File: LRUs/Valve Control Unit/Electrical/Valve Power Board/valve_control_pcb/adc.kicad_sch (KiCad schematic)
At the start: 8 parts, among them U37 AD7689BCP

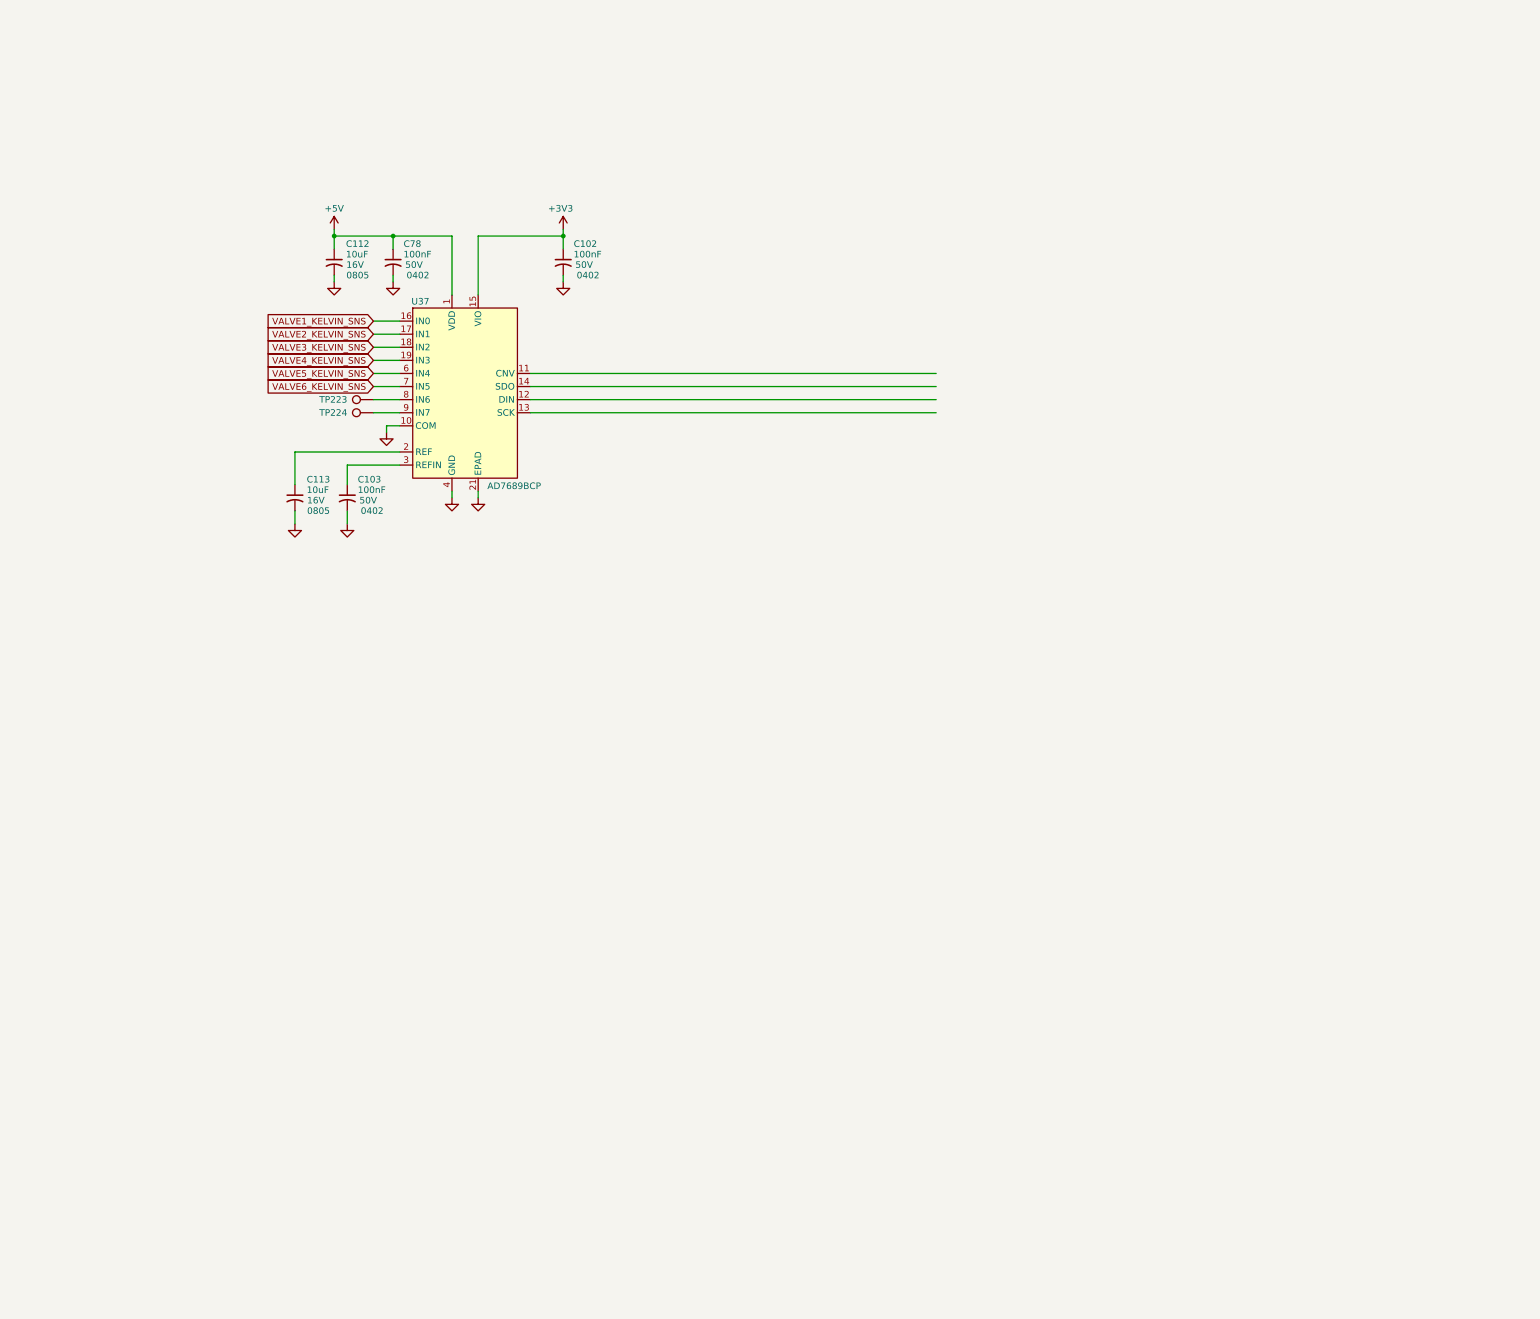
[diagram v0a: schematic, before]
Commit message: Committttt
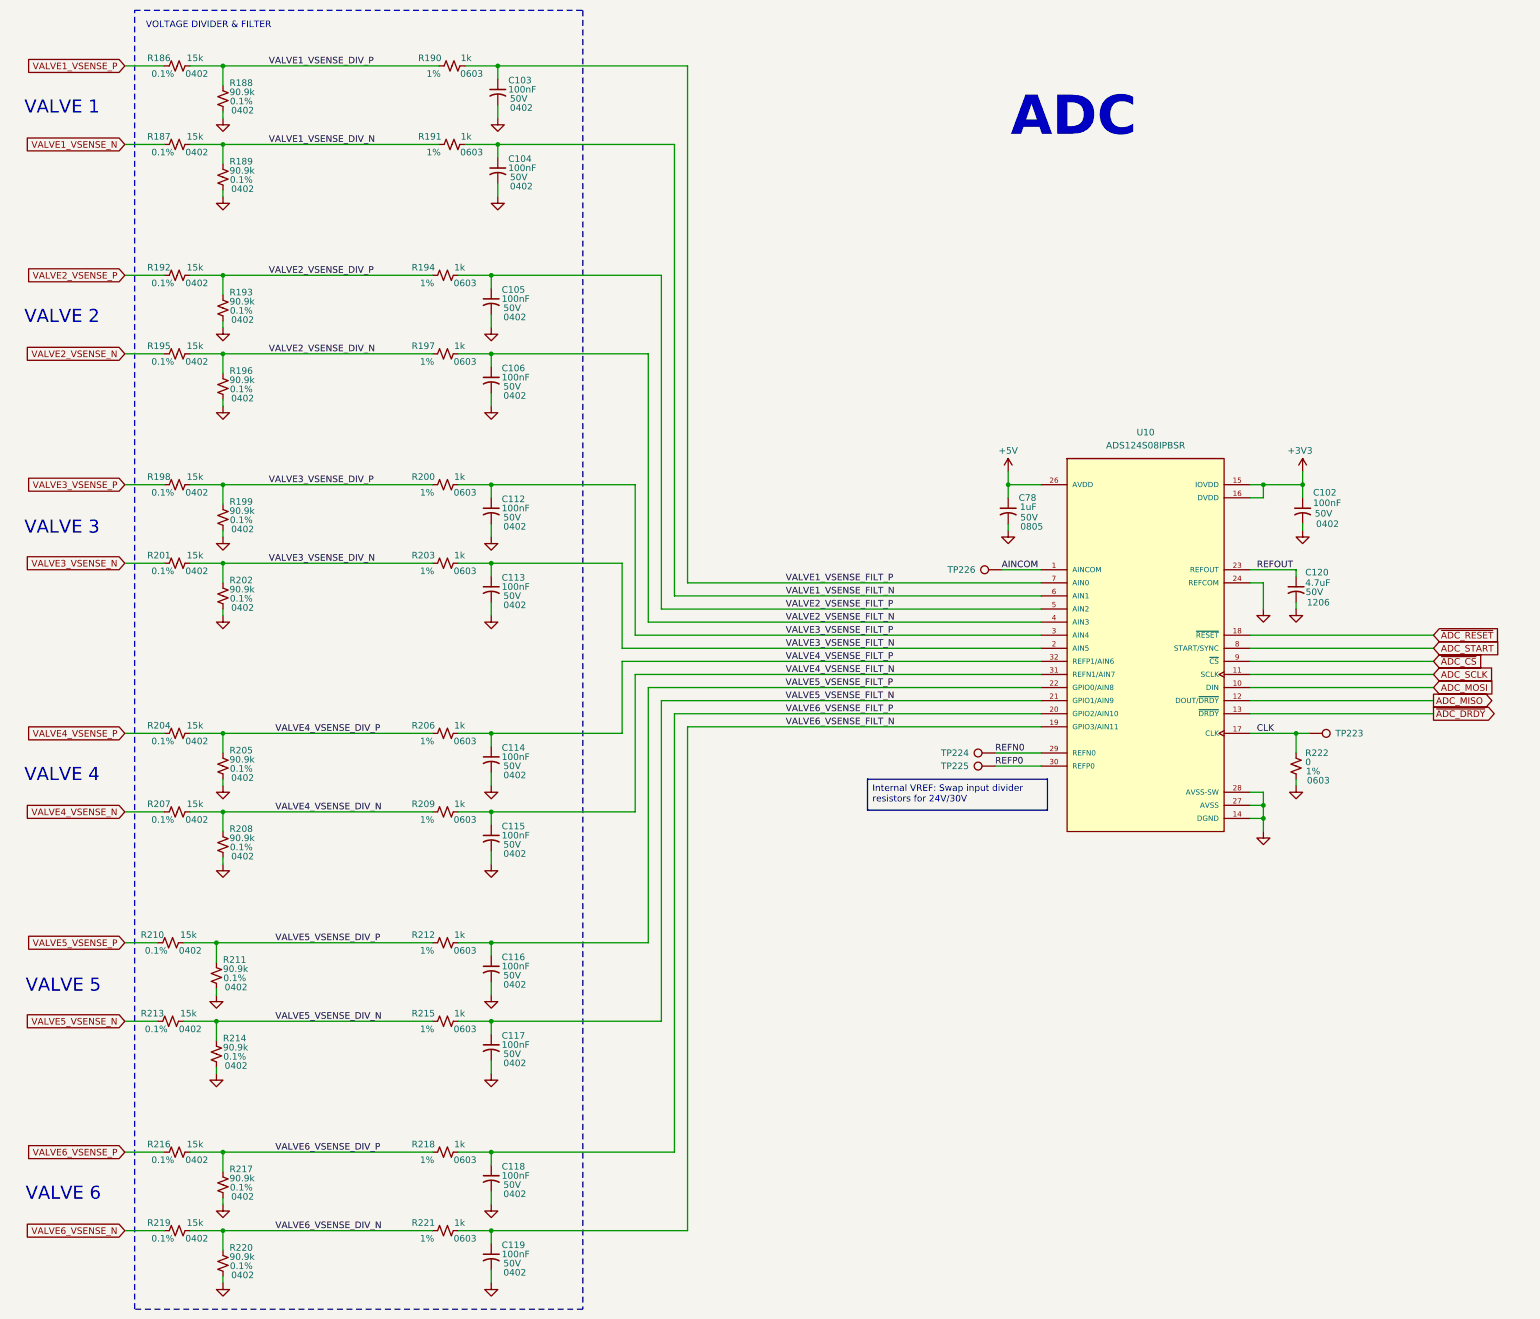
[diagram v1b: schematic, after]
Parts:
- removed U37: AD7689BCP, Package_CSP:LFCSP-20-1EP_4x4mm_P0.5mm_EP2.1x2.1mm, symbol Analog_ADC:AD7689xCP
- added C104, C105, C106, C114, C115, C116, C117, C118, C119: 100nF, Capacitor_SMD:C_0402_1005Metric, symbol Device:C_Small_US
- added C120: 4.7uF, Capacitor_SMD:C_1206_3216Metric, symbol Device:C_Small_US
- added R186, R187, R192, R195, R198, R201, R204, R207, R210, R213, R216, R219: 15k, Resistor_SMD:R_0402_1005Metric, symbol Device:R_Small_US
- added R188, R189, R193, R196, R199, R202, R205, R208, R211, R214, R217, R220: 90.9k, Resistor_SMD:R_0402_1005Metric, symbol Device:R_Small_US
- added R190, R191, R194, R197, R200, R203, R206, R209, R212, R215, R218, R221: 1k, Resistor_SMD:R_0603_1608Metric, symbol Device:R_Small_US
- added R222: 0, Resistor_SMD:R_0603_1608Metric, symbol Device:R_Small_US
- added TP225, TP226: TestPoint, TestPoint:TestPoint_Pad_D1.0mm, symbol Connector:TestPoint
- added U10: ADS124S08IPBSR, valve_pcb_footprints:QFP50P700X700X120-32N, symbol valve_pcb_symbols:ADS124S08IPBSR
- C112, C113: value 10uF -> 100nF; footprint Capacitor_SMD:C_0805_2012Metric -> Capacitor_SMD:C_0402_1005Metric; Footprint_Size 0805 -> 0402; JLCPCB Part # C95841 -> C307331; Vmax 16V -> 50V
- C78: value 100nF -> 1uF; footprint Capacitor_SMD:C_0402_1005Metric -> Capacitor_SMD:C_0805_2012Metric; Footprint_Size 0402 -> 0805; JLCPCB Part # C307331 -> C28323
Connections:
- net +3V3: now also U10.15 (IOVDD), U10.16 (DVDD)
- net +5V: now also U10.26 (AVDD); no longer C112.1
- net GND: now also C104.2, C105.2, C106.2, C114.2, C115.2, C116.2, C117.2, C118.2, C119.2, C120.2, R188.1, R189.1, R193.1, R196.1, R199.1, R202.1, R205.1, R208.1, R211.1, R214.1, R217.1, R220.1, R222.1, U10.14 (DGND), U10.24 (REFCOM), U10.27 (AVSS), U10.28 (AVSS-SW)
- net VALVE3_VSENSE_FILT_N: now reaches C113.1
- net VALVE3_VSENSE_FILT_N: now also R203.1, U10.2 (AIN5)
- net VALVE1_VSENSE_FILT_P: now reaches C103.1
- net VALVE1_VSENSE_FILT_P: now also R190.1, U10.7 (AIN0)
- net CLK: now reaches TP223.1
- net CLK: now also R222.2, U10.17 (CLK)
- net REFN0: now reaches TP224.1
- net REFN0: now also U10.29 (REFN0)
- new net ADC_MISO: U10.12 (DOUT/~{DRDY})
- new net ADC_MOSI: U10.10 (DIN)
- new net ADC_SCLK: U10.11 (SCLK)
- new net ADC_START: U10.8 (START/SYNC)
- new net AINCOM: TP226.1, U10.1 (AINCOM)
- new net REFOUT: C120.1, U10.23 (REFOUT)
- new net REFP0: TP225.1, U10.30 (REFP0)
- new net VALVE1_VSENSE_DIV_N: R187.1, R189.2, R191.2
- new net VALVE1_VSENSE_DIV_P: R186.1, R188.2, R190.2
- new net VALVE1_VSENSE_FILT_N: C104.1, R191.1, U10.6 (AIN1)
- new net VALVE1_VSENSE_N: R187.2
- new net VALVE1_VSENSE_P: R186.2
- new net VALVE2_VSENSE_DIV_N: R195.1, R196.2, R197.2
- new net VALVE2_VSENSE_DIV_P: R192.1, R193.2, R194.2
- new net VALVE2_VSENSE_FILT_N: C106.1, R197.1, U10.4 (AIN3)
- new net VALVE2_VSENSE_FILT_P: C105.1, R194.1, U10.5 (AIN2)
- new net VALVE2_VSENSE_N: R195.2
- new net VALVE2_VSENSE_P: R192.2
- new net VALVE3_VSENSE_DIV_N: R201.1, R202.2, R203.2
- new net VALVE3_VSENSE_DIV_P: R198.1, R199.2, R200.2
- new net VALVE3_VSENSE_FILT_P: C112.1, R200.1, U10.3 (AIN4)
- new net VALVE3_VSENSE_N: R201.2
- new net VALVE3_VSENSE_P: R198.2
- new net VALVE4_VSENSE_DIV_N: R207.1, R208.2, R209.2
- new net VALVE4_VSENSE_DIV_P: R204.1, R205.2, R206.2
- new net VALVE4_VSENSE_FILT_N: C115.1, R209.1, U10.31 (REFN1/AIN7)
- new net VALVE4_VSENSE_FILT_P: C114.1, R206.1, U10.32 (REFP1/AIN6)
- new net VALVE4_VSENSE_N: R207.2
- new net VALVE4_VSENSE_P: R204.2
- new net VALVE5_VSENSE_DIV_N: R213.1, R214.2, R215.2
- new net VALVE5_VSENSE_DIV_P: R210.1, R211.2, R212.2
- new net VALVE5_VSENSE_FILT_N: C117.1, R215.1, U10.21 (GPIO1/AIN9)
- new net VALVE5_VSENSE_FILT_P: C116.1, R212.1, U10.22 (GPIO0/AIN8)
- new net VALVE5_VSENSE_N: R213.2
- new net VALVE5_VSENSE_P: R210.2
- new net VALVE6_VSENSE_DIV_N: R219.1, R220.2, R221.2
- new net VALVE6_VSENSE_DIV_P: R216.1, R217.2, R218.2
- new net VALVE6_VSENSE_FILT_N: C119.1, R221.1, U10.19 (GPIO3/AIN11)
- new net VALVE6_VSENSE_FILT_P: C118.1, R218.1, U10.20 (GPIO2/AIN10)
- new net VALVE6_VSENSE_N: R219.2
- new net VALVE6_VSENSE_P: R216.2
- new net ~{ADC_CS}: U10.9 (~{CS})
- new net ~{ADC_DRDY}: U10.13 (~{DRDY})
- new net ~{ADC_RESET}: U10.18 (~{RESET})
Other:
- note added: "ADC"
- note added: "VALVE 1"
- note added: "VALVE 2"
- note added: "VALVE 3"
- note added: "VALVE 4"
- note added: "VALVE 5"
- note added: "VALVE 6"
- note added: "VOLTAGE DIVIDER & FILTER"
- title: (none) -> ADC
